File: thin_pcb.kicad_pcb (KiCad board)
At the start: 2 copper layers, 95.2 x 95.2 mm, 190 parts, among them J01 Conn_01x02, J02 Conn_01x02, J04 Conn_01x02, J06 Conn_01x02, J07 Conn_01x02, J08 Conn_01x02, J1 USB_B_Micro, J11 Conn_01x03, J12 Conn_01x03, J13 Conn_01x03, J14 Conn_01x03, J15 Conn_01x03, J16 Conn_01x03, J17 Conn_01x03, J18 Conn_01x03, J2 AudioJack4_Ground, J21 Conn_01x07, J22 Conn_01x07, J23 Conn_01x07, J24 Conn_01x07, J25 Conn_01x07, J26 Conn_01x07, J27 Conn_01x07, J28 Conn_01x07, J3 AudioJack4_Ground, J31 Conn_01x07, J32 Conn_01x07, J33 Conn_01x07, J34 Conn_01x07, J35 Conn_01x07, J36 Conn_01x07, J37 Conn_01x07, J38 Conn_01x07, J4 Conn_01x06, J41 Conn_01x04, J42 Conn_01x04, J43 Conn_01x04, J44 Conn_01x04, J45 Conn_01x04, J46 Conn_01x04, J47 Conn_01x04, J48 Conn_01x04, J5 Conn_01x06, J51 Conn_01x01, J52 Conn_01x01, J53 Conn_01x01, J54 Conn_01x01, J55 Conn_01x01, J56 Conn_01x01, J57 Conn_01x01, J58 Conn_01x01, J6 Conn_02x02, J7 Conn_01x02, SW11 SW_Push, SW12 SW_Push, SW13 SW_Push, SW14 SW_Push, SW15 SW_Push, SW21 SW_Push, SW22 SW_Push, SW23 SW_Push, SW24 SW_Push, SW25 SW_Push, SW252 SW_Push, SW31 SW_Push, SW32 SW_Push, SW33 SW_Push, SW34 SW_Push, SW35 SW_Push, SW41 SW_Push, SW42 SW_Push, SW422 SW_Push, SW43 SW_Push, SW44 SW_Push, SW45 SW_Push, SW452 SW_Push, SW51 SW_Push, SW52 SW_Push, SW522 SW_Push, SW53 SW_Push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

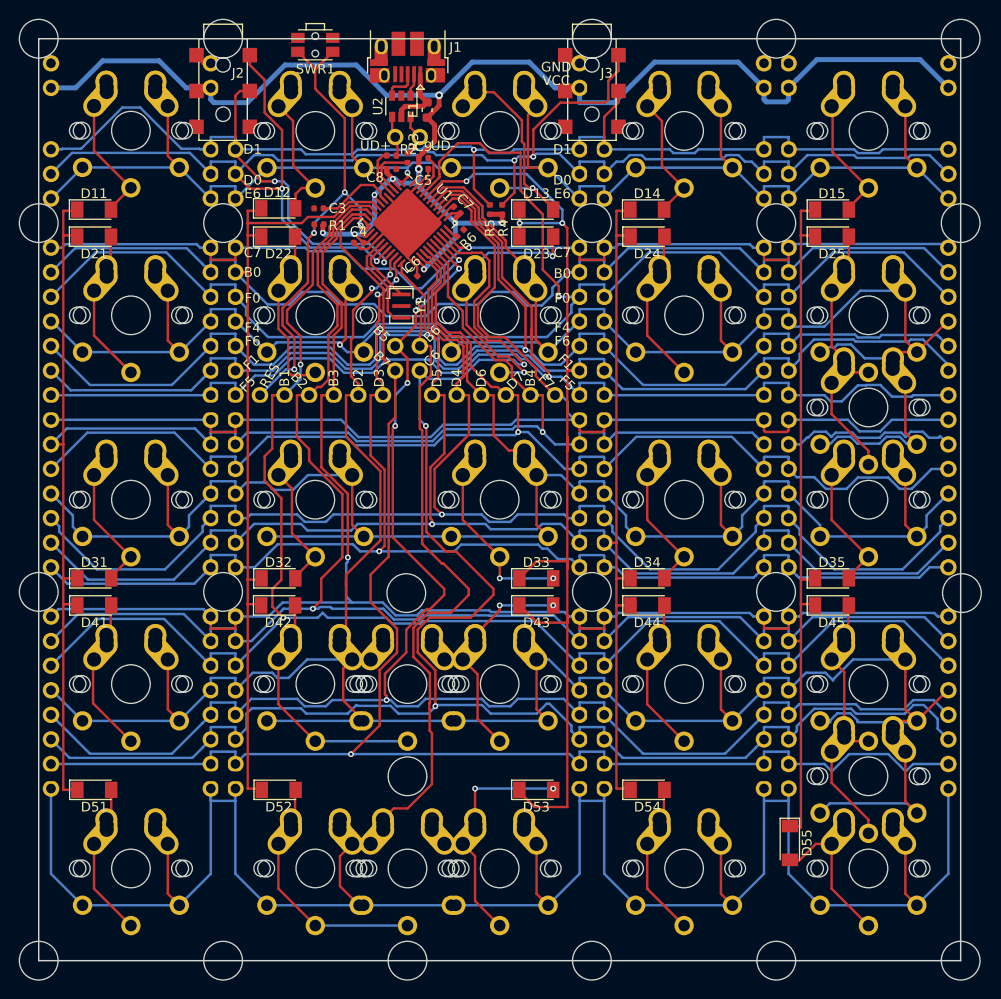
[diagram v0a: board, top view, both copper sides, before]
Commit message: fixes
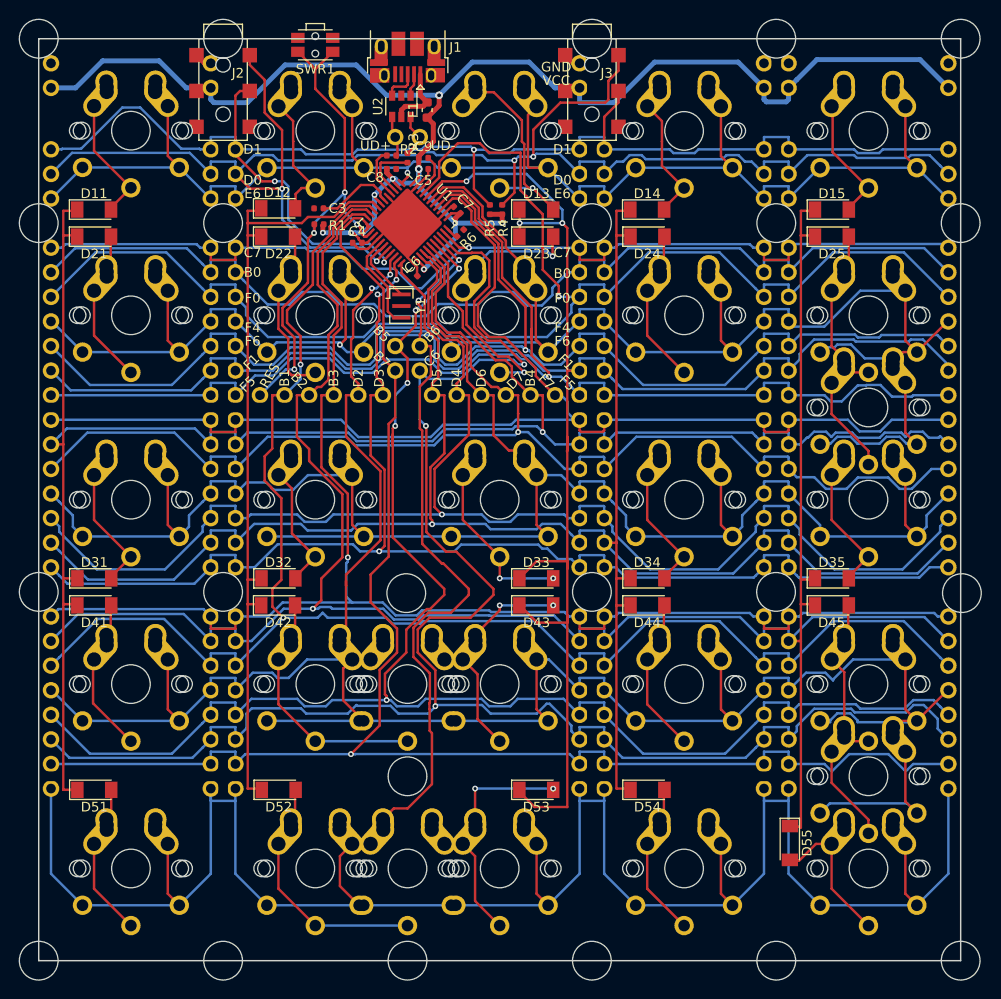
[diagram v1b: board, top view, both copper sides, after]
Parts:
- removed the ? at (105.4, 81.9) (x2)
- added ? (x2): , , F.Cu at (105.4, 81.9)
- moved C4 0.13 mm to (84.4, 80.1)
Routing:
- net B4: track 198.4 -> 200.8 mm
- net GND: track 35.1 -> 32.9 mm
